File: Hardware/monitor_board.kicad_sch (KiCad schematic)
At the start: 2 parts

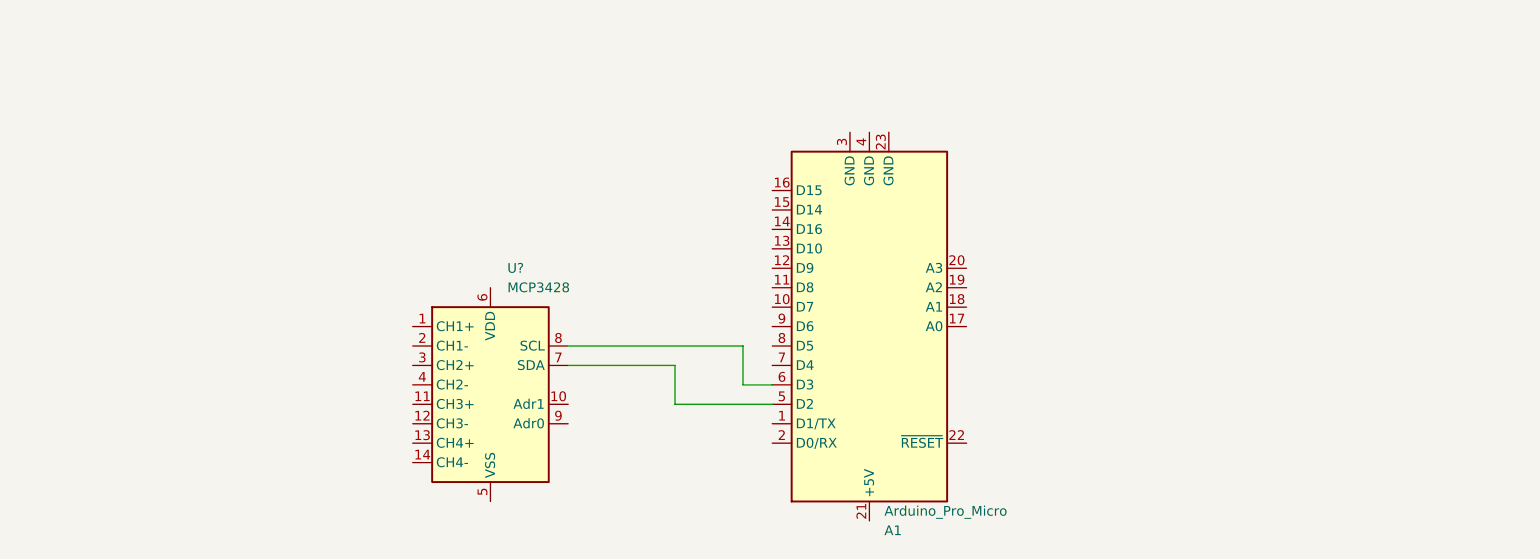
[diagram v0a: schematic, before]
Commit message: Add files via upload
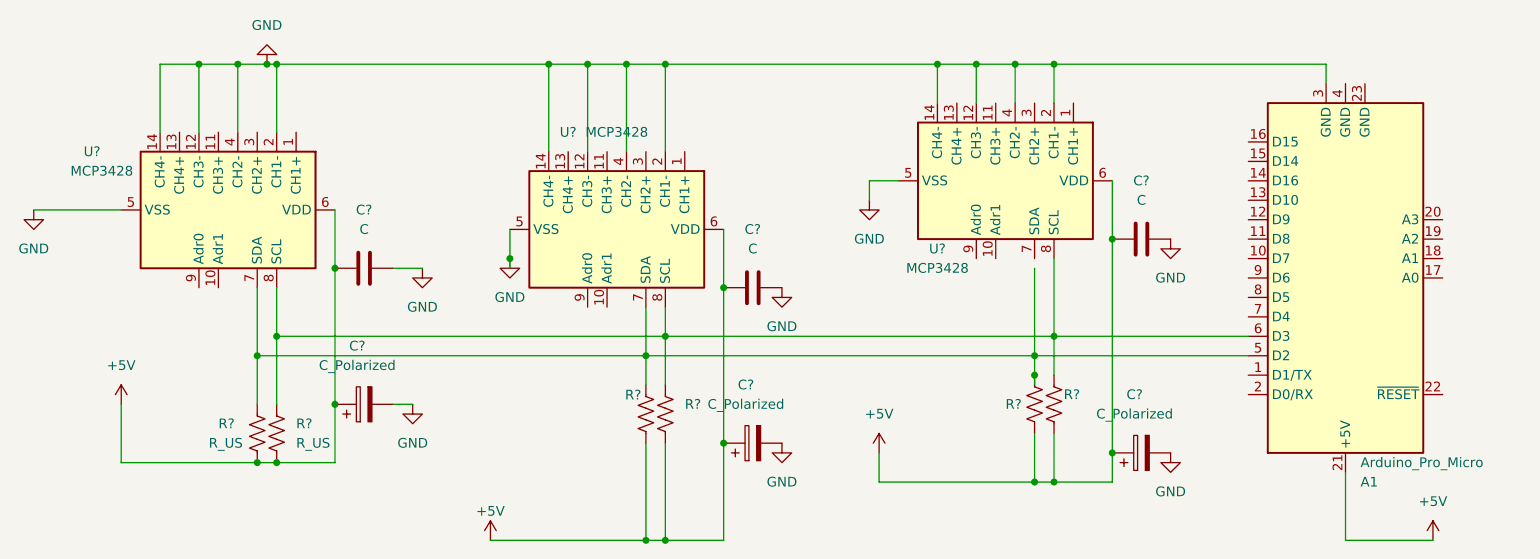
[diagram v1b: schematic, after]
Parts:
- added C? (x3): C, symbol Device:C
- added C? (x3): C_Polarized, symbol Device:C_Polarized
- added R? (x6): R_US, symbol Device:R_US
- added U? (x2): MCP3428, symbol Analog_ADC:MCP3428
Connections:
- net GND: now reaches U?.12 (CH3-)
- net GND: now also A1.3 (GND), U?.14 (CH4-), U?.2 (CH1-), U?.4 (CH2-), U?.5 (VSS), C?.2, C?.2, C?.2, C?.2, C?.2, C?.2, U?.12 (CH3-), U?.12 (CH3-), U?.14 (CH4-), U?.14 (CH4-), U?.2 (CH1-), U?.2 (CH1-), U?.4 (CH2-), U?.4 (CH2-), U?.5 (VSS), U?.5 (VSS)
- net +5V: now reaches U?.6 (VDD)
- net +5V: now also A1.21 (+5V), C?.1, C?.1, C?.1, C?.1, C?.1, C?.1, R?.1, R?.2, R?.2, R?.2, R?.2, R?.2, U?.6 (VDD), U?.6 (VDD)
- net at A1.5 (D2): now also R?.1, R?.1, R?.2, U?.7 (SDA), U?.7 (SDA); no longer U?.7 (SDA)
- net at A1.6 (D3), U?.8 (SCL): now also R?.1, R?.1, R?.1, U?.8 (SCL), U?.8 (SCL)
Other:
- moved on the sheet: A1, U?
